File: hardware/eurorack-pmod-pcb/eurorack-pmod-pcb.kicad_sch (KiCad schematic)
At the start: 77 parts, among them J1 EURORACK_PWR, J10 PJ301BM, J2 PMOD_CONN, J3 PJ301BM, J4 PJ301BM, J5 PJ301BM, J6 PJ301BM, J7 PJ301BM, J8 PJ301BM, J9 PJ301BM, U1 LM1117-3.3, U2 TL072, U3 TL072, U4 TL072, U5 AK4619VN, U6 TL072, U7 TL072

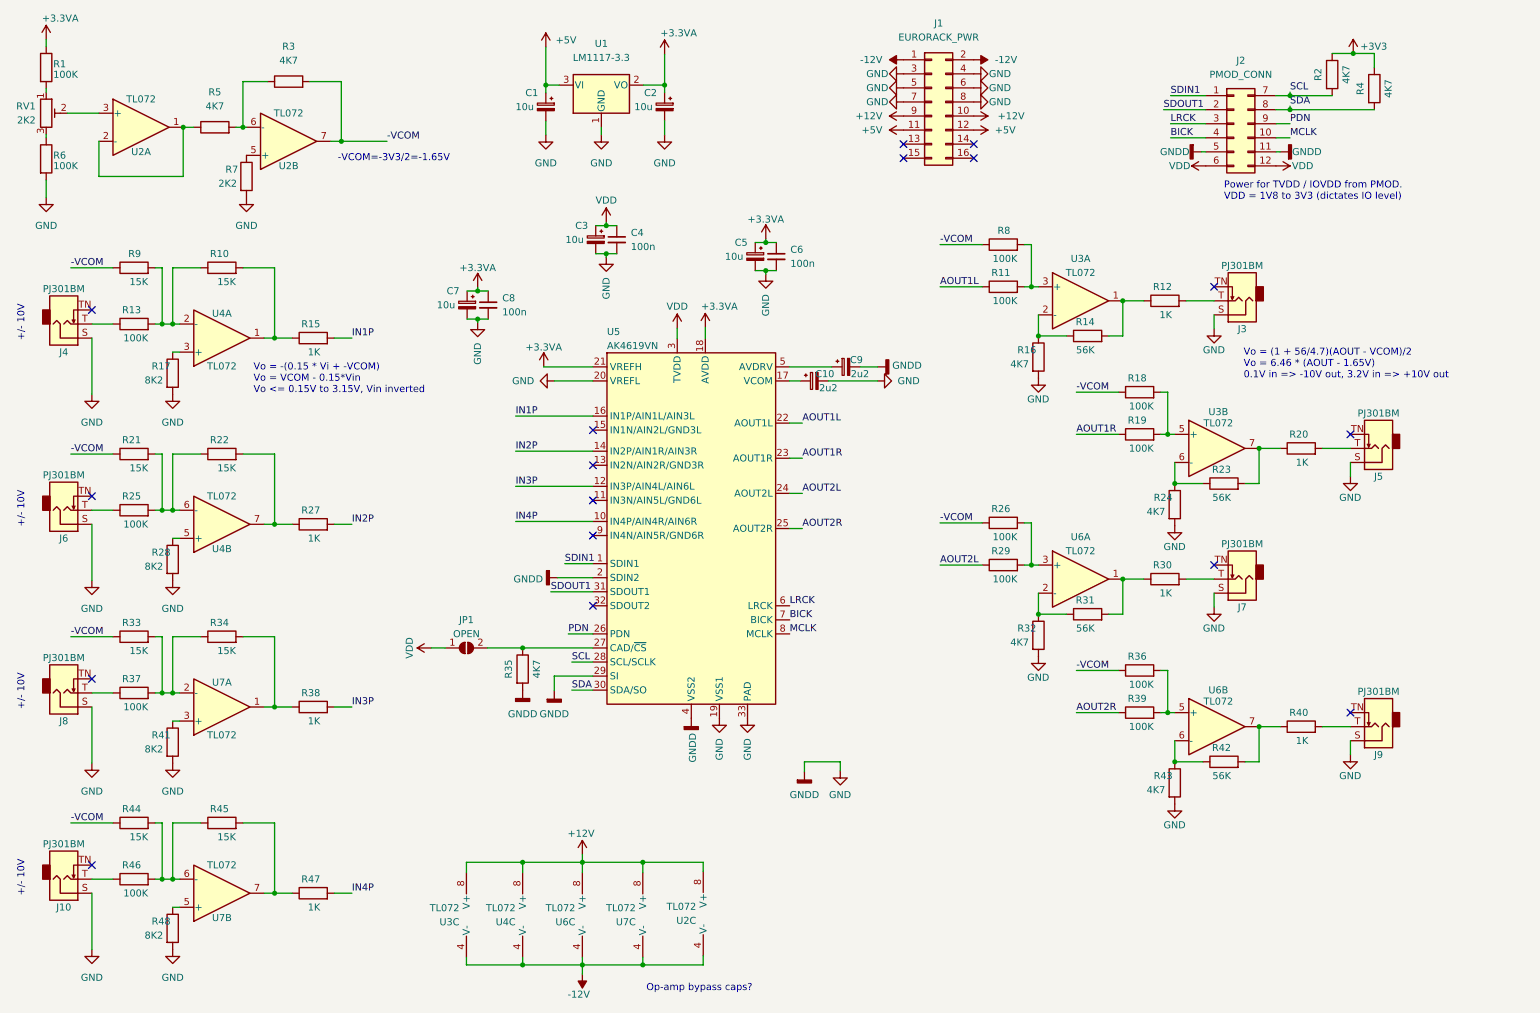
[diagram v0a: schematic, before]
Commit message: Finish schematic capture, ERC, footprints
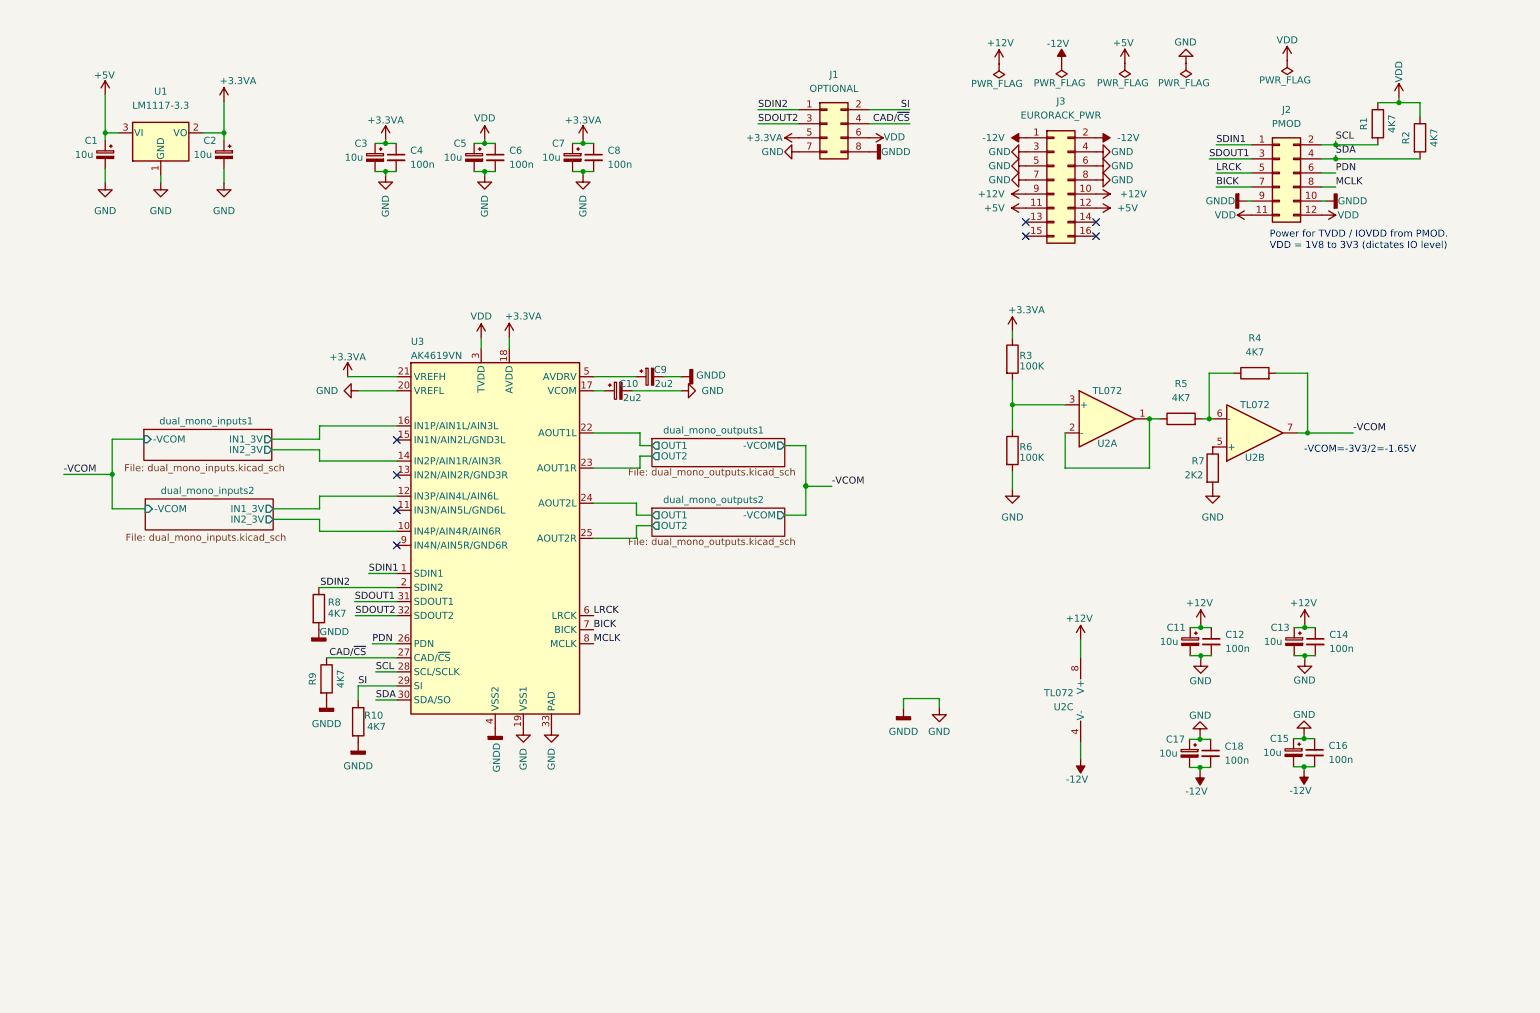
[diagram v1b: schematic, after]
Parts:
- removed J10, J3, J4, J5, J6, J7, J8, J9: PJ301BM, AudioJacks:Jack_3.5mm_QingPu_WQP-PJ301BM_Vertical, symbol Connector:AudioJack2_SwitchT
- removed J2: PMOD_CONN, symbol Connector_Generic:Conn_02x06_Top_Bottom
- removed JP1: OPEN, Resistor_SMD:R_0603_1608Metric, symbol Jumper:SolderJumper_2_Open
- removed R11, R13, R18, R19, R25, R26, R29, R36, R37, R39, R46: 100K, Resistor_SMD:R_0603_1608Metric, symbol Device:R
- removed R12, R15, R20, R27, R30, R38, R40, R47: 1K, Resistor_SMD:R_0603_1608Metric, symbol Device:R
- removed R14, R23, R31, R42: 56K, Resistor_SMD:R_0603_1608Metric, symbol Device:R
- removed R16, R24, R32, R43: 4K7, Resistor_SMD:R_0603_1608Metric, symbol Device:R
- removed R17, R28, R41, R48: 8K2, Resistor_SMD:R_0603_1608Metric, symbol Device:R
- removed R21, R22, R33, R34, R44, R45, R9: 15K, Resistor_SMD:R_0603_1608Metric, symbol Device:R
- removed RV1: 2K2, symbol Device:R_Potentiometer_Trim
- removed unit 3 of U2
- removed U3, U4, U7: TL072, Package_SO:SOIC-8_3.9x4.9mm_P1.27mm, symbol Amplifier_Operational:TL072
- removed unit 1 of U6
- removed unit 2 of U6
- added C11, C13, C15, C17: 10u, Capacitor_Tantalum_SMD:CP_EIA-3216-10_Kemet-I, symbol Device:C_Polarized_Small
- added C12, C14, C16, C18: 100n, Capacitor_SMD:C_0603_1608Metric, symbol Device:C_Small
- added J1: OPTIONAL, Connector_PinHeader_2.54mm:PinHeader_2x04_P2.54mm_Vertical, symbol Connector_Generic:Conn_02x04_Odd_Even
- added J2: PMOD, Connector_PinHeader_2.54mm:PinHeader_2x06_P2.54mm_Vertical, symbol Connector_Generic:Conn_02x06_Odd_Even
- C1, C10, C2, C9: footprint (none) -> Capacitor_Tantalum_SMD:CP_EIA-3216-10_Kemet-I
- C3: renamed from C7; footprint (none) -> Capacitor_Tantalum_SMD:CP_EIA-3216-10_Kemet-I
- C5: renamed from C3; footprint (none) -> Capacitor_Tantalum_SMD:CP_EIA-3216-10_Kemet-I
- C7: renamed from C5; footprint (none) -> Capacitor_Tantalum_SMD:CP_EIA-3216-10_Kemet-I
- J3: renamed from J1; footprint (none) -> Connector_PinHeader_2.54mm:PinHeader_2x08_P2.54mm_Vertical
- R10: value 15K -> 4K7
- R8: value 100K -> 4K7
- renumbered C8 to C4, C4 to C6, C6 to C8, R2 to R1, R4 to R2, R1 to R3, R3 to R4, R35 to R9, U6 to U2, U5 to U3
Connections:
- net +3V3 is gone; now on net VDD: R1.1, R2.1
- net +12V: now also C11.1, C12.1, C13.1, C14.1
- net +3.3VA: now also J1.5 (Pin_5)
- net -12V: now also C15.2, C16.2, C17.2, C18.2
- net -VCOM: no longer R8.1
- net BICK: now also J2.7 (Pin_7)
- net GND: now also R10.2, R8.2, C11.2, C12.2, C13.2, C14.2, C15.1, C16.1, C17.1, C18.1, J1.7 (Pin_7), J1.8 (Pin_8), J2.10 (Pin_10), J2.9 (Pin_9); no longer U3.2 (SDIN2), U3.29 (SI)
- net LRCK: now also J2.5 (Pin_5)
- net MCLK: now also J2.8 (Pin_8)
- net PDN: now also J2.6 (Pin_6)
- net SCL: now also J2.2 (Pin_2)
- net SDA: now also J2.4 (Pin_4)
- net SDIN1: now also J2.1 (Pin_1)
- net SDOUT1: now also J2.3 (Pin_3)
- net VDD: now also J1.6 (Pin_6), J2.11 (Pin_11), J2.12 (Pin_12)
- net at U2.3 (+): now also R3.2, R6.1
- net SI: now reaches R10.1
- net SI: now also U3.29 (SI), J1.2 (Pin_2)
- net CAD/~{CS}: now reaches R9.1, U3.27 (CAD/~{CS})
- net CAD/~{CS}: now also J1.4 (Pin_4)
- net SDOUT2: now reaches U3.32 (SDOUT2)
- net SDOUT2: now also J1.3 (Pin_3)
- net AOUT1L renamed dual_mono_outputs1/OUT1
- net AOUT1R renamed dual_mono_outputs1/OUT2
- net AOUT2L renamed dual_mono_outputs2/OUT1
- net AOUT2R renamed dual_mono_outputs2/OUT2
- net IN1P renamed dual_mono_inputs1/IN1_3V
- net IN2P renamed dual_mono_inputs1/IN2_3V
- net IN3P renamed dual_mono_inputs2/IN1_3V
- net IN4P renamed dual_mono_inputs2/IN2_3V
- new net SDIN2: J1.1 (Pin_1), R8.1, U3.2 (SDIN2)
- no-connect marks 17 -> 8
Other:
- added sheet dual_mono_inputs1 (dual_mono_inputs.kicad_sch)
- added sheet dual_mono_inputs2 (dual_mono_inputs.kicad_sch)
- added sheet dual_mono_outputs1 (dual_mono_outputs.kicad_sch)
- added sheet dual_mono_outputs2 (dual_mono_outputs.kicad_sch)
- note removed: "+/- 10V"
- note removed: "Op-amp bypass caps?"
- note removed: "Vo = (1 + 56/4.7)(AOUT - VCOM)/2 Vo = 6.46 * (AOUT - 1.65V) 0.1V in => -10V out, 3.2V in => +10V out"
- note removed: "Vo = -(0.15 * Vi + -VCOM) Vo = VCOM - 0.15*Vin Vo <= 0.15V to 3.15V, Vin inverted"
- moved on the sheet: C1, C10, C2, C3, C4, C5, C6, C7, C8, C9, J3, R1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
